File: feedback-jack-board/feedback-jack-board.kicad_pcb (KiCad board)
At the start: 2 copper layers, 80 x 37 mm, 12 parts, among them J1 Out, J2 Ret, J3 In, J4 Snd, J5 908140508, J6 Barrel_Jack_Switch

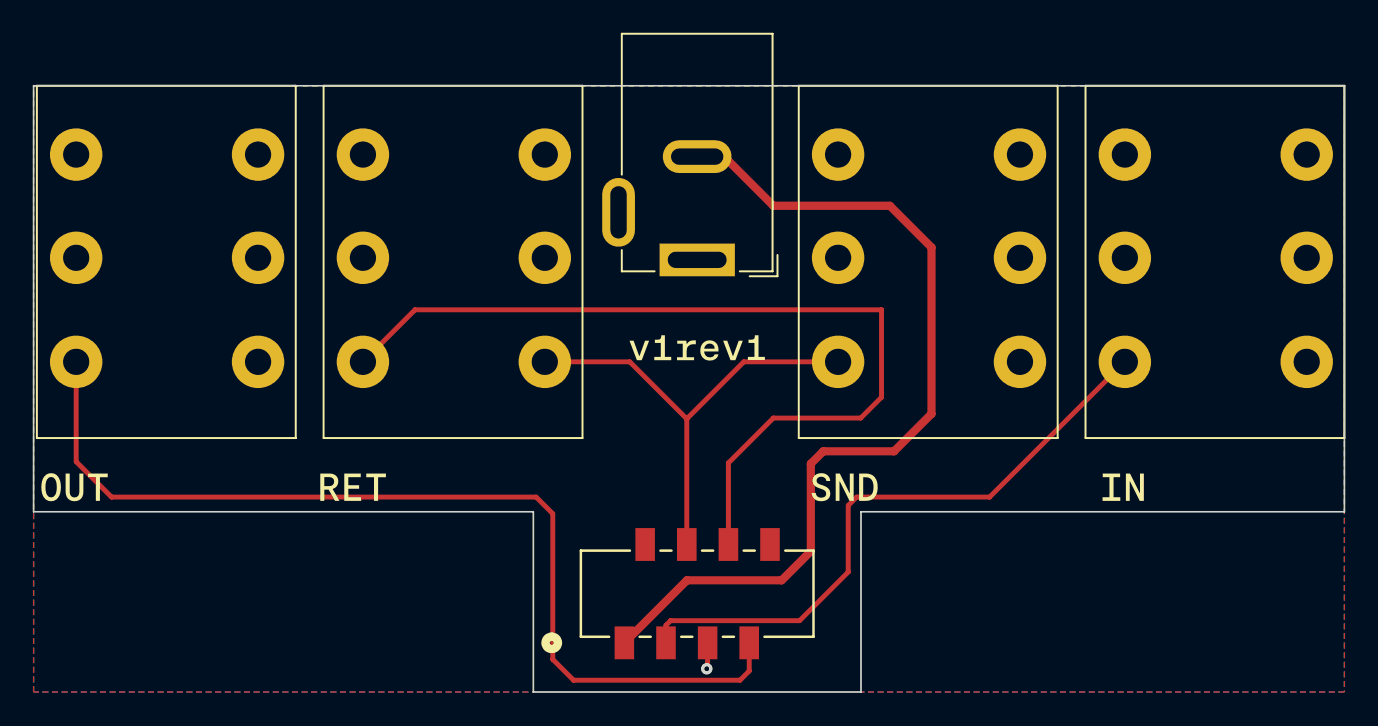
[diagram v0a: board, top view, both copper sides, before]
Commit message: rev2 wip start
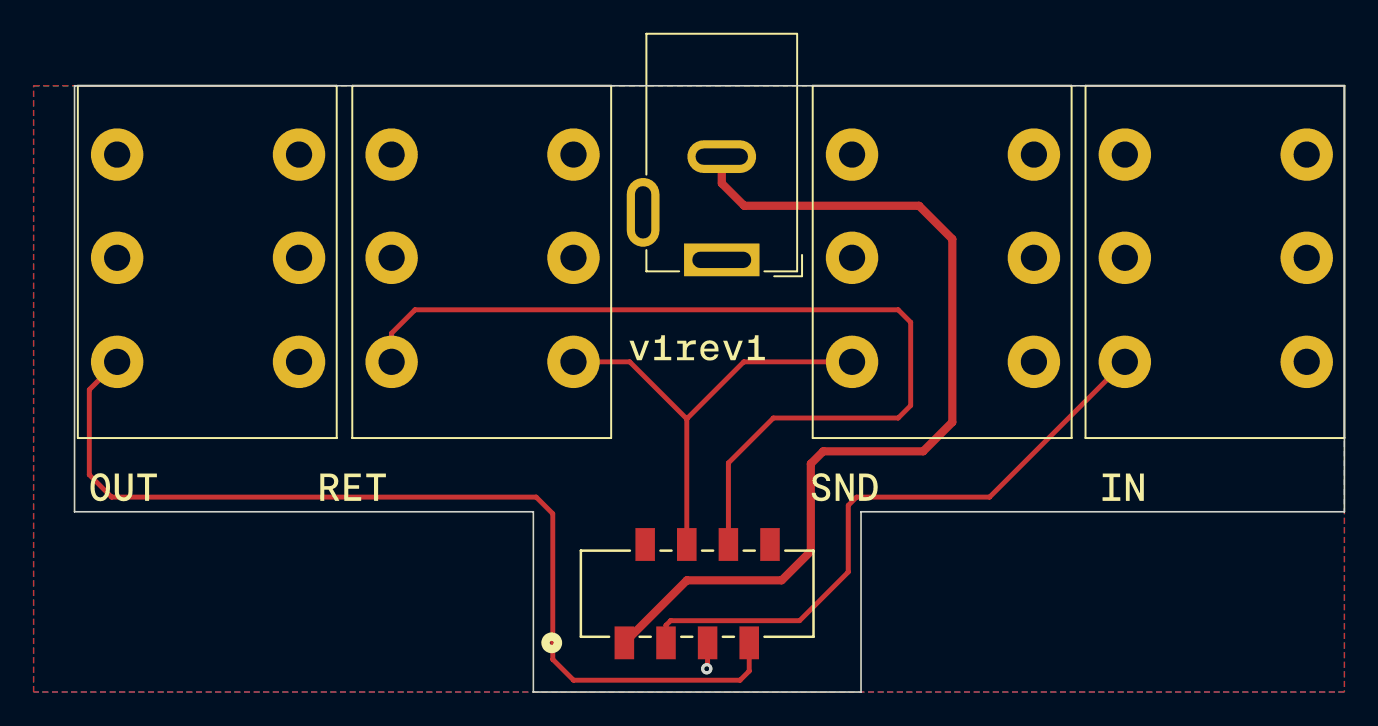
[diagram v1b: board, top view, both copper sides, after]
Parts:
- moved kibuzzard-67A4F113 3.00 mm to (65.0, 69.5)
- moved J1 2.50 mm to (71.5, 45.0)
- moved J2 1.75 mm to (88.2, 45.0)
- moved J6 1.50 mm to (101.5, 55.6)
- moved J4 0.85 mm to (116.3, 45.0)
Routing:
- net /Ret: track 54.3 -> 57.0 mm
- net /Jack9V: track 54.4 -> 57.0 mm
- net /Snd: track 28.5 -> 27.6 mm
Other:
- board size 80 x 37 mm -> 77.5 x 37 mm
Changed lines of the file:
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@@
   (net 19 "unconnected-(J6-Pad3)")
   (footprint "Connector_BarrelJack:BarrelJack_GCT_DCJ200-10-A_Horizontal" (layer "F.Cu")
-    (at 100 55.626 180)
+    (at 101.5 55.626 180)
     (descr "Barrel jack connector (5.5 mm outer diameter, 2.05 inner diameter ), https://gct.co/files/drawings/dcj200-10.pdf")
     (tags "connector barrel jack")
@@
   )
   (footprint "kibuzzard-67A4F113" (layer "F.Cu")
-    (at 62 69.5)
+    (at 65 69.5)
     (descr "Generated with KiBuzzard")
     (tags "kb_params=eyJBbGlnbm1lbnRDaG9pY2UiOiAiQ2VudGVyIiwgIkNhcExlZnRDaG9pY2UiOiAiIiwgIkNhcFJpZ2h0Q2hvaWNlIjogIiIsICJGb250Q29tYm9Cb3giOiAiTW9kZXJhdC1Nb25vLU1lZGl1bSIsICJIZWlnaHRDdHJsIjogIjEuNSIsICJMYXllckNvbWJvQm94IjogIkYuU2lsa1MiLCAiTXVsdGlMaW5lVGV4dCI6ICJPVVQiLCAiUGFkZGluZ0JvdHRvbUN0cmwiOiAiNSIsICJQYWRkaW5nTGVmdEN0cmwiOiAiNSIsICJQYWRkaW5nUmlnaHRDdHJsIjogIjUiLCAiUGFkZGluZ1RvcEN0cmwiOiAiNSIsICJXaWR0aEN0cmwiOiAiMS41In0=")
@@
   )
   (footprint "Tayda-A6446-6-35mm-Compact-PCB-Mounted-Jack:tayda-A6446-6mm35-jack-pcb-compact" (layer "F.Cu")
-    (at 69 45 90)
+    (at 71.5 45 90)
     (property "Sheetfile" "feedback-jack-board.kicad_sch")
     (property "Sheetname" "")
@@
   )
   (footprint "Tayda-A6446-6-35mm-Compact-PCB-Mounted-Jack:tayda-A6446-6mm35-jack-pcb-compact" (layer "F.Cu")
-    (at 115.5 45 90)
+    (at 116.35 45 90)
     (property "Sheetfile" "feedback-jack-board.kicad_sch")
     (property "Sheetname" "")
@@
   )
   (footprint "Tayda-A6446-6-35mm-Compact-PCB-Mounted-Jack:tayda-A6446-6mm35-jack-pcb-compact" (layer "F.Cu")
-    (at 86.5 45 90)
+    (at 88.25 45 90)
     (property "Sheetfile" "feedback-jack-board.kicad_sch")
     (property "Sheetname" "")
@@
   )
   (gr_line (start 110 71) (end 139.5 71) (layer "Edge.Cuts") (width 0.1))
-  (gr_line (start 59.5 45) (end 139.5 45) (layer "Edge.Cuts") (width 0.1))
-  (gr_line (start 90 71) (end 59.5 71) (layer "Edge.Cuts") (width 0.1))
+  (gr_line (start 62 45) (end 139.5 45) (layer "Edge.Cuts") (width 0.1))
+  (gr_line (start 90 71) (end 62 71) (layer "Edge.Cuts") (width 0.1))
   (gr_line (start 110 82) (end 90 82) (layer "Edge.Cuts") (width 0.1))
-  (gr_line (start 59.5 71) (end 59.5 45) (layer "Edge.Cuts") (width 0.1))
+  (gr_line (start 62 71) (end 62 45) (layer "Edge.Cuts") (width 0.1))
   (gr_line (start 139.5 45) (end 139.5 71) (layer "Edge.Cuts") (width 0.1))
   (gr_line (start 110 82) (end 110 71) (layer "Edge.Cuts") (width 0.1))
@@
   (segment (start 100.635 78.998099) (end 100.635 80.5295) (width 0.3) (layer "F.Cu") (net 3))
   (via (at 100.584 80.5805) (size 0.7) (drill 0.3) (layers "F.Cu" "B.Cu") (net 3))
+  (segment (start 92.456 81.28) (end 91.186 80.01) (width 0.3) (layer "F.Cu") (net 4))
+  (segment (start 103.175 78.998099) (end 103.175 80.721) (width 0.3) (layer "F.Cu") (net 4))
+  (segment (start 62.9 63.55) (end 64.6 61.85) (width 0.3) (layer "F.Cu") (net 4))
+  (segment (start 90.17 70.104) (end 64.262 70.104) (width 0.3) (layer "F.Cu") (net 4))
+  (segment (start 64.262 70.104) (end 62.9 68.742) (width 0.3) (layer "F.Cu") (net 4))
   (segment (start 91.186 80.01) (end 91.186 71.12) (width 0.3) (layer "F.Cu") (net 4))
-  (segment (start 103.175 78.998099) (end 103.175 80.721) (width 0.3) (layer "F.Cu") (net 4))
   (segment (start 102.616 81.28) (end 92.456 81.28) (width 0.3) (layer "F.Cu") (net 4))
-  (segment (start 64.262 70.104) (end 62.1 67.942) (width 0.3) (layer "F.Cu") (net 4))
-  (segment (start 62.1 67.942) (end 62.1 61.85) (width 0.3) (layer "F.Cu") (net 4))
+  (segment (start 91.186 71.12) (end 90.17 70.104) (width 0.3) (layer "F.Cu") (net 4))
+  (segment (start 62.9 68.742) (end 62.9 63.55) (width 0.3) (layer "F.Cu") (net 4))
   (segment (start 103.175 80.721) (end 102.616 81.28) (width 0.3) (layer "F.Cu") (net 4))
-  (segment (start 92.456 81.28) (end 91.186 80.01) (width 0.3) (layer "F.Cu") (net 4))
-  (segment (start 91.186 71.12) (end 90.17 70.104) (width 0.3) (layer "F.Cu") (net 4))
-  (segment (start 90.17 70.104) (end 64.262 70.104) (width 0.3) (layer "F.Cu") (net 4))
-  (segment (start 82.776 58.674) (end 111.252 58.674) (width 0.3) (layer "F.Cu") (net 8))
-  (segment (start 111.252 58.674) (end 111.252 64.008) (width 0.3) (layer "F.Cu") (net 8))
-  (segment (start 109.982 65.278) (end 104.648 65.278) (width 0.3) (layer "F.Cu") (net 8))
-  (segment (start 79.6 61.85) (end 82.776 58.674) (width 0.3) (layer "F.Cu") (net 8))
+  (segment (start 112.268 65.278) (end 104.648 65.278) (width 0.3) (layer "F.Cu") (net 8))
+  (segment (start 101.905 68.021) (end 101.905 72.998098) (width 0.3) (layer "F.Cu") (net 8))
   (segment (start 104.648 65.278) (end 101.905 68.021) (width 0.3) (layer "F.Cu") (net 8))
-  (segment (start 101.905 68.021) (end 101.905 72.998098) (width 0.3) (layer "F.Cu") (net 8))
-  (segment (start 111.252 64.008) (end 109.982 65.278) (width 0.3) (layer "F.Cu") (net 8))
+  (segment (start 112.268 58.674) (end 113.03 59.436) (width 0.3) (layer "F.Cu") (net 8))
+  (segment (start 113.03 59.436) (end 113.03 64.516) (width 0.3) (layer "F.Cu") (net 8))
+  (segment (start 81.35 61.85) (end 81.35 60.1) (width 0.3) (layer "F.Cu") (net 8))
+  (segment (start 113.03 64.516) (end 112.268 65.278) (width 0.3) (layer "F.Cu") (net 8))
+  (segment (start 81.35 60.1) (end 82.776 58.674) (width 0.3) (layer "F.Cu") (net 8))
+  (segment (start 82.776 58.674) (end 112.268 58.674) (width 0.3) (layer "F.Cu") (net 8))
+  (segment (start 95.886 61.85) (end 92.45 61.85) (width 0.3) (layer "F.Cu") (net 9))
+  (segment (start 102.844 61.85) (end 109.45 61.85) (width 0.3) (layer "F.Cu") (net 9))
   (segment (start 99.365 65.329) (end 99.365 72.998098) (width 0.3) (layer "F.Cu") (net 9))
   (segment (start 99.365 65.329) (end 102.844 61.85) (width 0.3) (layer "F.Cu") (net 9))
   (segment (start 95.886 61.85) (end 99.365 65.329) (width 0.3) (layer "F.Cu") (net 9))
-  (segment (start 90.7 61.85) (end 95.886 61.85) (width 0.3) (layer "F.Cu") (net 9))
-  (segment (start 102.844 61.85) (end 108.6 61.85) (width 0.3) (layer "F.Cu") (net 9))
   (segment (start 109.22 70.612) (end 109.728 70.104) (width 0.3) (layer "F.Cu") (net 12))
   (segment (start 98.377201 77.644799) (end 106.251201 77.644799) (width 0.3) (layer "F.Cu") (net 12))
@@
   (segment (start 106.251201 77.644799) (end 109.22 74.676) (width 0.3) (layer "F.Cu") (net 12))
   (segment (start 117.846 70.104) (end 126.1 61.85) (width 0.3) (layer "F.Cu") (net 12))
-  (segment (start 107.696 67.31) (end 106.934 68.072) (width 0.5) (layer "F.Cu") (net 17))
-  (segment (start 105.156 75.184) (end 99.369099 75.184) (width 0.5) (layer "F.Cu") (net 17))
-  (segment (start 106.934 68.072) (end 106.934 73.406) (width 0.5) (layer "F.Cu") (net 17))
-  (segment (start 99.369099 75.184) (end 95.555 78.998099) (width 0.5) (layer "F.Cu") (net 17))
-  (segment (start 114.3 54.864) (end 114.3 65.024) (width 0.5) (layer "F.Cu") (net 17))
-  (segment (start 112.014 67.31) (end 107.696 67.31) (width 0.5) (layer "F.Cu") (net 17))
-  (segment (start 111.76 52.324) (end 114.3 54.864) (width 0.5) (layer "F.Cu") (net 17))
-  (segment (start 100 49.326) (end 101.65 49.326) (width 0.5) (layer "F.Cu") (net 17))
-  (segment (start 104.648 52.324) (end 111.76 52.324) (width 0.5) (layer "F.Cu") (net 17))
-  (segment (start 106.934 73.406) (end 105.156 75.184) (width 0.5) (layer "F.Cu") (net 17))
-  (segment (start 101.65 49.326) (end 104.648 52.324) (width 0.5) (layer "F.Cu") (net 17))
-  (segment (start 114.3 65.024) (end 112.014 67.31) (width 0.5) (layer "F.Cu") (net 17))
+  (segment (start 106.934 68.072) (end 107.696 67.31) (width 0.5) (layer "F.Cu") (net 17))
+  (segment (start 99.369099 75.184) (end 105.156 75.184) (width 0.5) (layer "F.Cu") (net 17))
+  (segment (start 102.87 52.324) (end 101.5 50.954) (width 0.5) (layer "F.Cu") (net 17))
+  (segment (start 113.792 67.31) (end 115.57 65.532) (width 0.5) (layer "F.Cu") (net 17))
+  (segment (start 107.696 67.31) (end 113.792 67.31) (width 0.5) (layer "F.Cu") (net 17))
+  (segment (start 113.538 52.324) (end 102.87 52.324) (width 0.5) (layer "F.Cu") (net 17))
+  (segment (start 115.57 65.532) (end 115.57 54.356) (width 0.5) (layer "F.Cu") (net 17))
+  (segment (start 95.555 78.998099) (end 99.369099 75.184) (width 0.5) (layer "F.Cu") (net 17))
+  (segment (start 115.57 54.356) (end 113.538 52.324) (width 0.5) (layer "F.Cu") (net 17))
+  (segment (start 105.156 75.184) (end 106.934 73.406) (width 0.5) (layer "F.Cu") (net 17))
+  (segment (start 101.5 50.954) (end 101.5 49.326) (width 0.5) (layer "F.Cu") (net 17))
+  (segment (start 106.934 73.406) (end 106.934 68.072) (width 0.5) (layer "F.Cu") (net 17))
   (zone (net 3) (net_name "/GND") (layers F&B.Cu) (hatch edge 0.508)
     (connect_pads (clearance 0.508))
